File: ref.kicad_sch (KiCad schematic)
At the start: 13 parts, among them Q1 Q_NPN_BCE, U4 ADR1000, U5 Opamp_Dual

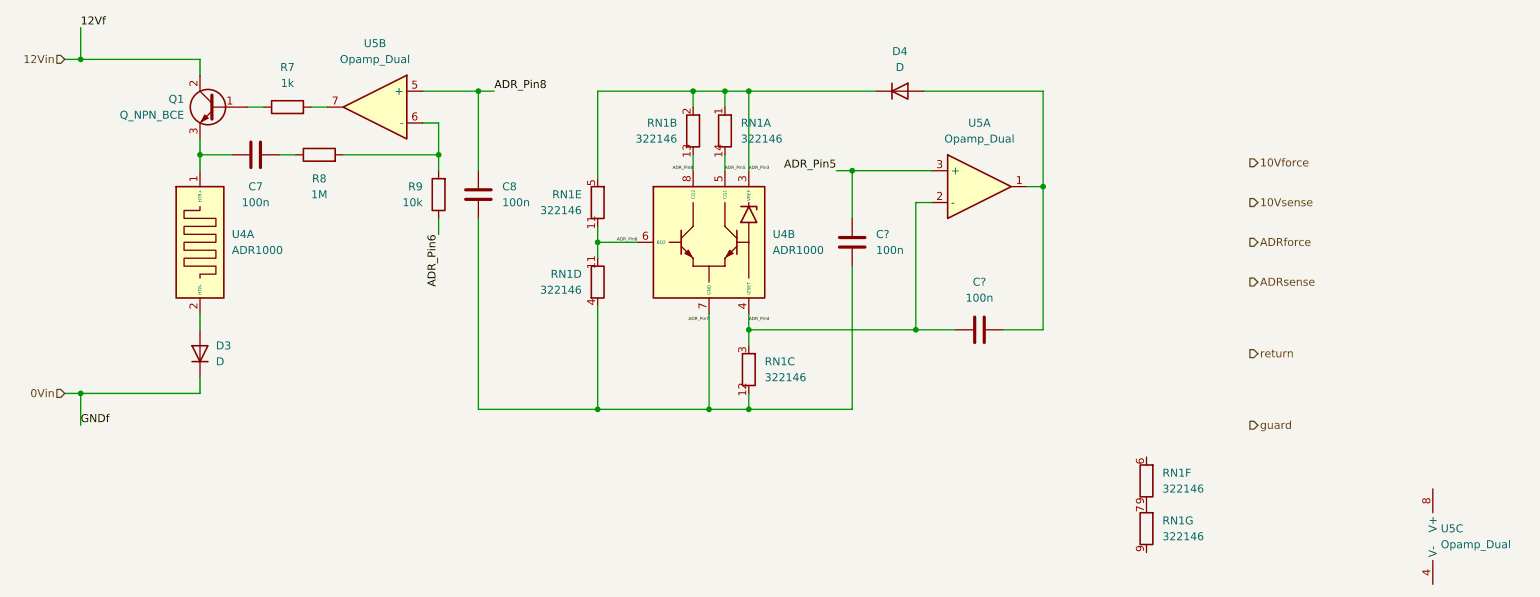
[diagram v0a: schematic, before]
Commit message: asdf
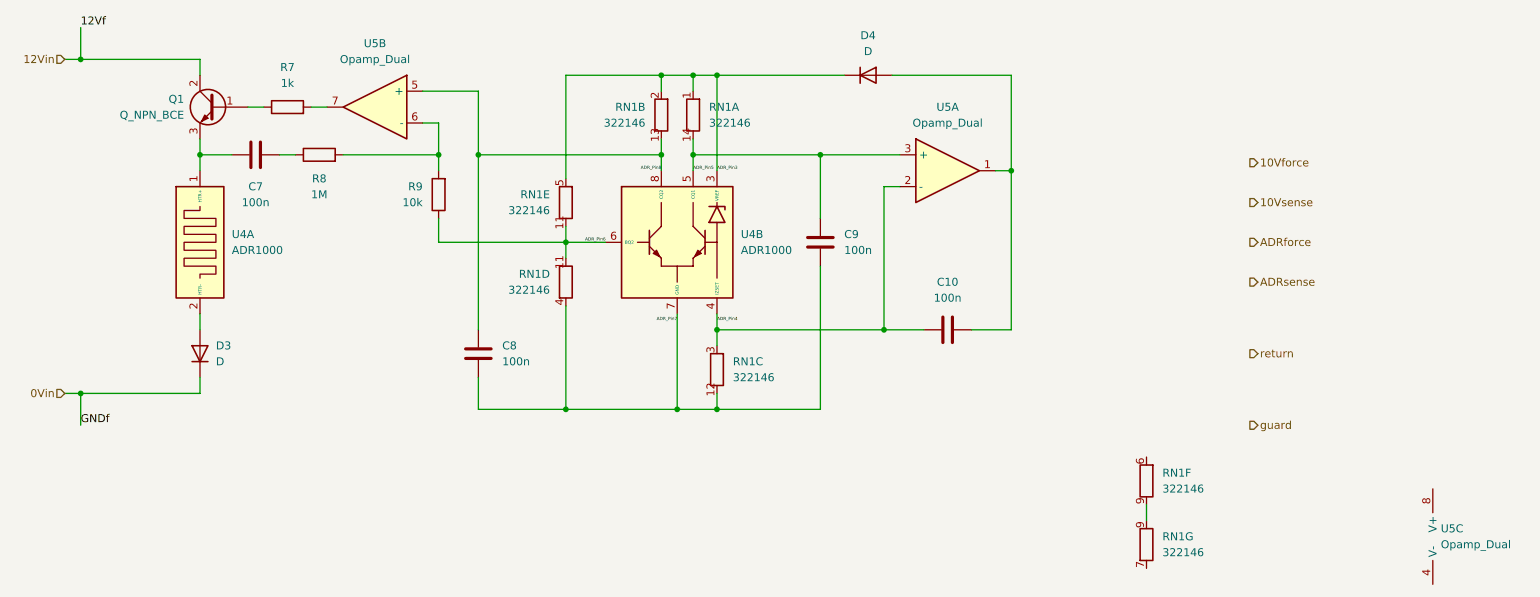
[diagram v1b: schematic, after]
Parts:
- gave numbers to parts that had none: 2
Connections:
- net at RN1.9 (R6.2): now also RN1.9 (R7.2); no longer RN1.7 (R7.1)
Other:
- moved on the sheet: C10, C8, C9, D4, RN1A, RN1B, RN1C, RN1D, RN1E, RN1G, U4B, U5A
